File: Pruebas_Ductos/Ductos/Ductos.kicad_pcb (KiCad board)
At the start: 2 copper layers, 26.7 x 53.3 mm, 4 parts, among them J1 Conn_01x04_Female, U1 SensordePresion

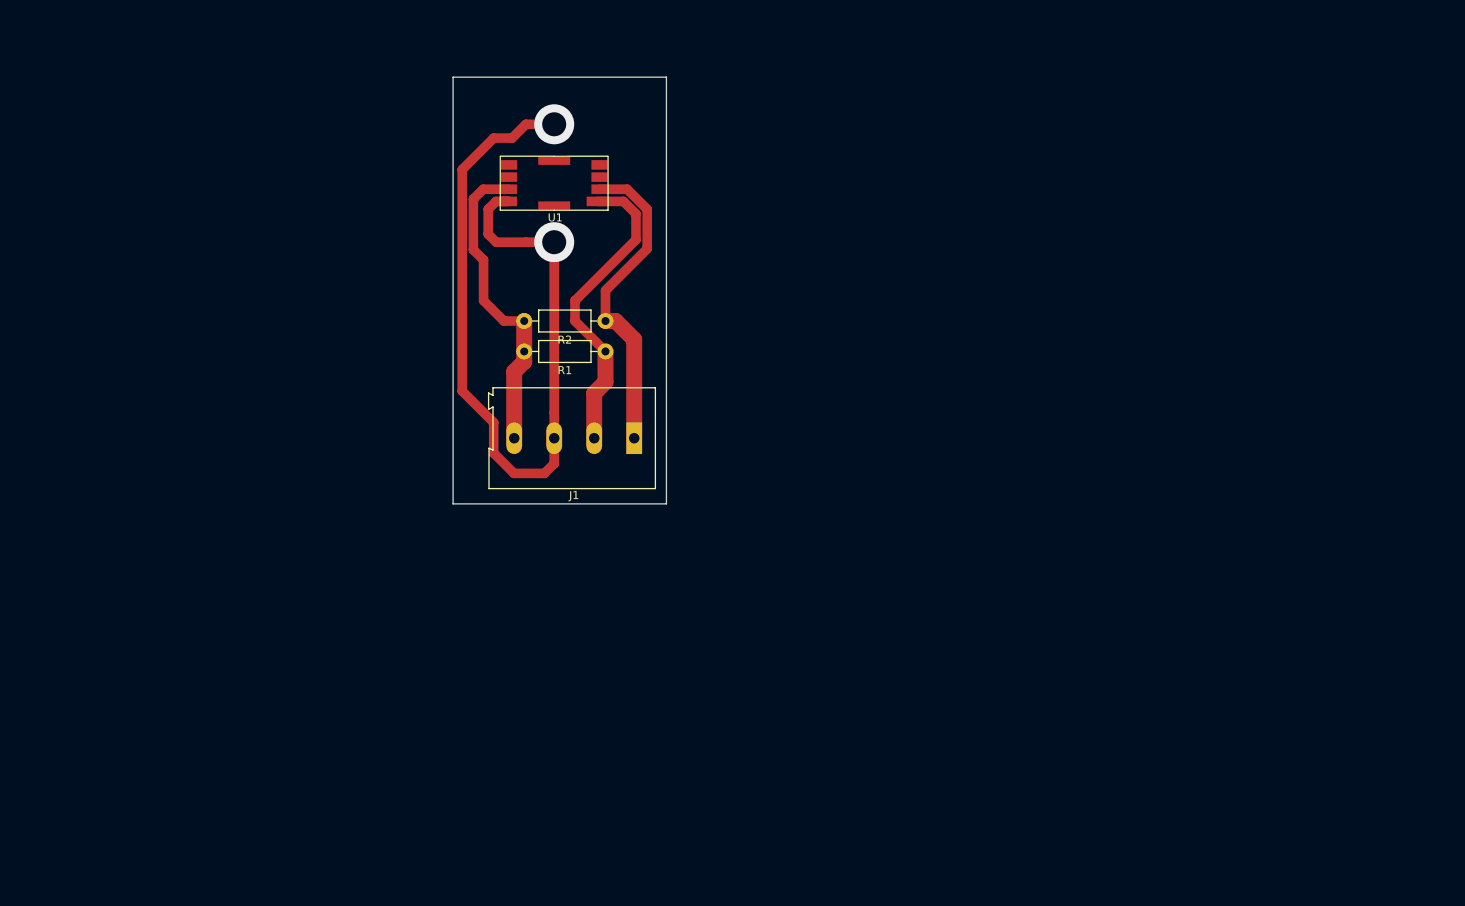
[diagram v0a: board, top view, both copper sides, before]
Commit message: niksd
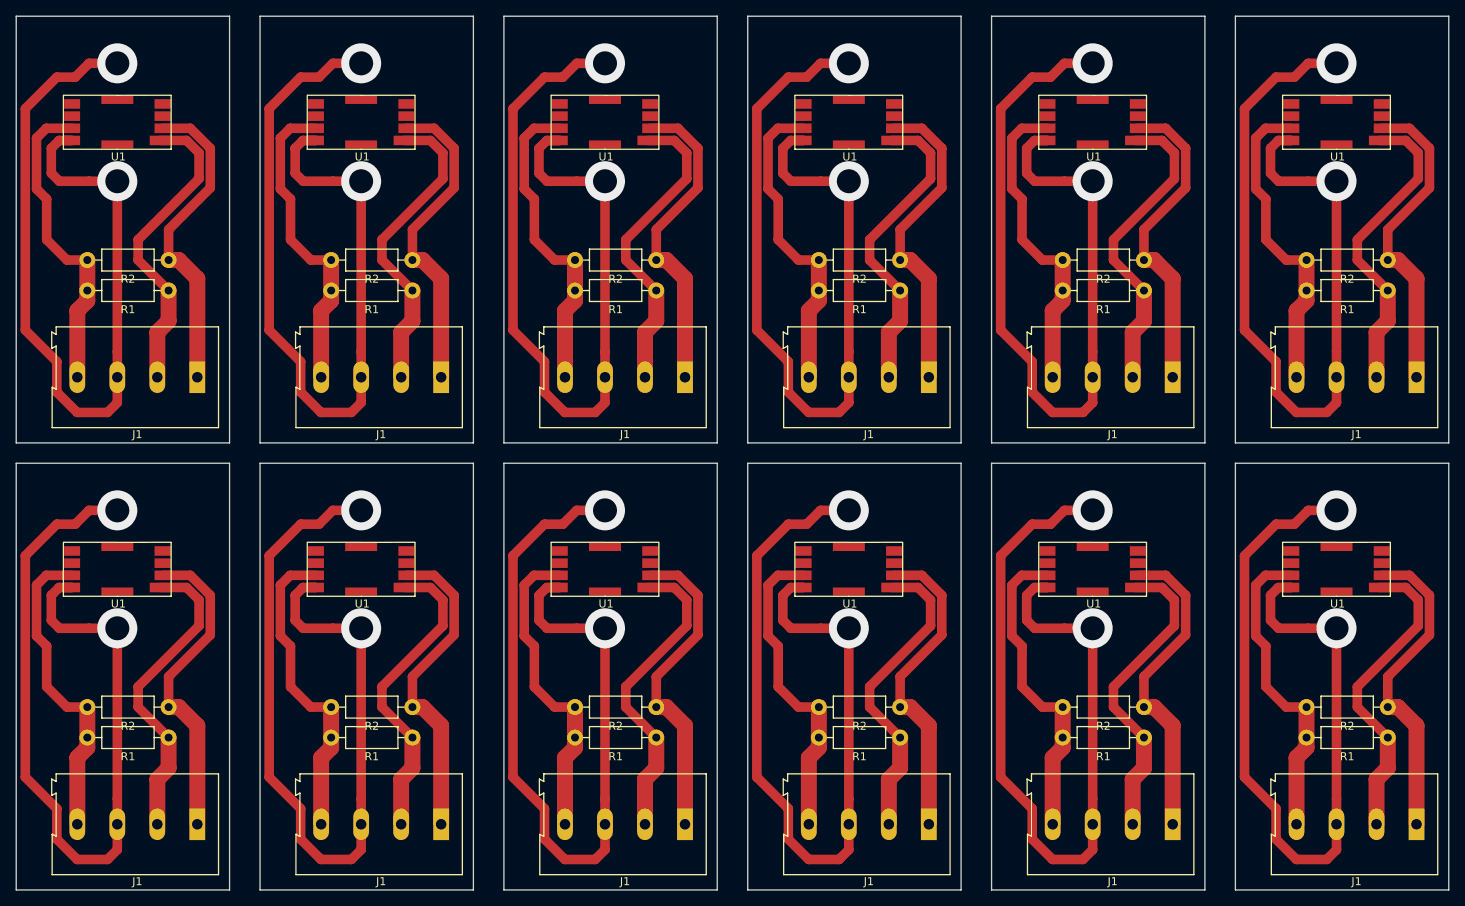
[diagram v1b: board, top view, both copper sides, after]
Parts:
- added J1: Conn_01x04_Female, TerminalBlock:TerminalBlock_Altech_AK300-4_P5.00mm, F.Cu at (176.3, 76.9)
- added J1: Conn_01x04_Female, TerminalBlock:TerminalBlock_Altech_AK300-4_P5.00mm, F.Cu at (115.3, 76.9)
- added J1: Conn_01x04_Female, TerminalBlock:TerminalBlock_Altech_AK300-4_P5.00mm, F.Cu at (84.9, 76.9)
- added J1: Conn_01x04_Female, TerminalBlock:TerminalBlock_Altech_AK300-4_P5.00mm, F.Cu at (206.8, 76.9)
- added J1: Conn_01x04_Female, TerminalBlock:TerminalBlock_Altech_AK300-4_P5.00mm, F.Cu at (206.8, 132.8)
- added J1: Conn_01x04_Female, TerminalBlock:TerminalBlock_Altech_AK300-4_P5.00mm, F.Cu at (176.3, 132.8)
- added J1: Conn_01x04_Female, TerminalBlock:TerminalBlock_Altech_AK300-4_P5.00mm, F.Cu at (145.8, 132.8)
- added J1: Conn_01x04_Female, TerminalBlock:TerminalBlock_Altech_AK300-4_P5.00mm, F.Cu at (145.8, 76.9)
- added J1: Conn_01x04_Female, TerminalBlock:TerminalBlock_Altech_AK300-4_P5.00mm, F.Cu at (115.3, 132.8)
- added J1: Conn_01x04_Female, TerminalBlock:TerminalBlock_Altech_AK300-4_P5.00mm, F.Cu at (84.9, 132.8)
- added J1: Conn_01x04_Female, TerminalBlock:TerminalBlock_Altech_AK300-4_P5.00mm, F.Cu at (54.4, 132.8)
- added R1: R, Resistor_THT:R_Axial_DIN0207_L6.3mm_D2.5mm_P10.16mm_Horizontal, F.Cu at (203.2, 66.0)
- added R1: R, Resistor_THT:R_Axial_DIN0207_L6.3mm_D2.5mm_P10.16mm_Horizontal, F.Cu at (111.8, 66.0)
- added R1: R, Resistor_THT:R_Axial_DIN0207_L6.3mm_D2.5mm_P10.16mm_Horizontal, F.Cu at (81.3, 66.0)
- added R1: R, Resistor_THT:R_Axial_DIN0207_L6.3mm_D2.5mm_P10.16mm_Horizontal, F.Cu at (172.7, 66.0)
- added R1: R, Resistor_THT:R_Axial_DIN0207_L6.3mm_D2.5mm_P10.16mm_Horizontal, F.Cu at (172.7, 121.9)
- added R1: R, Resistor_THT:R_Axial_DIN0207_L6.3mm_D2.5mm_P10.16mm_Horizontal, F.Cu at (203.2, 121.9)
- added R1: R, Resistor_THT:R_Axial_DIN0207_L6.3mm_D2.5mm_P10.16mm_Horizontal, F.Cu at (142.2, 121.9)
- added R1: R, Resistor_THT:R_Axial_DIN0207_L6.3mm_D2.5mm_P10.16mm_Horizontal, F.Cu at (142.2, 66.0)
- added R1: R, Resistor_THT:R_Axial_DIN0207_L6.3mm_D2.5mm_P10.16mm_Horizontal, F.Cu at (111.8, 121.9)
- added R1: R, Resistor_THT:R_Axial_DIN0207_L6.3mm_D2.5mm_P10.16mm_Horizontal, F.Cu at (81.3, 121.9)
- added R1: R, Resistor_THT:R_Axial_DIN0207_L6.3mm_D2.5mm_P10.16mm_Horizontal, F.Cu at (50.8, 121.9)
- added R2: R, Resistor_THT:R_Axial_DIN0207_L6.3mm_D2.5mm_P10.16mm_Horizontal, F.Cu at (203.2, 62.2)
- added R2: R, Resistor_THT:R_Axial_DIN0207_L6.3mm_D2.5mm_P10.16mm_Horizontal, F.Cu at (111.8, 62.2)
- added R2: R, Resistor_THT:R_Axial_DIN0207_L6.3mm_D2.5mm_P10.16mm_Horizontal, F.Cu at (81.3, 62.2)
- added R2: R, Resistor_THT:R_Axial_DIN0207_L6.3mm_D2.5mm_P10.16mm_Horizontal, F.Cu at (172.7, 62.2)
- added R2: R, Resistor_THT:R_Axial_DIN0207_L6.3mm_D2.5mm_P10.16mm_Horizontal, F.Cu at (203.2, 118.1)
- added R2: R, Resistor_THT:R_Axial_DIN0207_L6.3mm_D2.5mm_P10.16mm_Horizontal, F.Cu at (172.7, 118.1)
- added R2: R, Resistor_THT:R_Axial_DIN0207_L6.3mm_D2.5mm_P10.16mm_Horizontal, F.Cu at (142.2, 118.1)
- added R2: R, Resistor_THT:R_Axial_DIN0207_L6.3mm_D2.5mm_P10.16mm_Horizontal, F.Cu at (142.2, 62.2)
- added R2: R, Resistor_THT:R_Axial_DIN0207_L6.3mm_D2.5mm_P10.16mm_Horizontal, F.Cu at (111.8, 118.1)
- added R2: R, Resistor_THT:R_Axial_DIN0207_L6.3mm_D2.5mm_P10.16mm_Horizontal, F.Cu at (81.3, 118.1)
- added R2: R, Resistor_THT:R_Axial_DIN0207_L6.3mm_D2.5mm_P10.16mm_Horizontal, F.Cu at (50.8, 118.1)
- added U1: SensordePresion, Boards:SensorPresion, F.Cu at (196.8, 47.8)
- added U1: SensordePresion, Boards:SensorPresion, F.Cu at (105.3, 47.8)
- added U1: SensordePresion, Boards:SensorPresion, F.Cu at (74.9, 47.8)
- added U1: SensordePresion, Boards:SensorPresion, F.Cu at (166.3, 47.8)
- added U1: SensordePresion, Boards:SensorPresion, F.Cu at (196.8, 103.7)
- added U1: SensordePresion, Boards:SensorPresion, F.Cu at (166.3, 103.7)
- added U1: SensordePresion, Boards:SensorPresion, F.Cu at (135.8, 103.7)
- added U1: SensordePresion, Boards:SensorPresion, F.Cu at (135.8, 47.8)
- added U1: SensordePresion, Boards:SensorPresion, F.Cu at (105.3, 103.7)
- added U1: SensordePresion, Boards:SensorPresion, F.Cu at (74.9, 103.7)
- added U1: SensordePresion, Boards:SensorPresion, F.Cu at (44.4, 103.7)
- moved J1 55.1 mm to (54.4, 76.9)
- moved R1 55.1 mm to (50.8, 66.0)
- moved R2 55.1 mm to (50.8, 62.2)
- moved U1 55.1 mm to (44.4, 47.8)
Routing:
- net (no net): track 0.00 -> 2439.8 mm, vias 0 -> 22
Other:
- board size 26.7 x 53.3 mm -> 179.1 x 109.2 mm
